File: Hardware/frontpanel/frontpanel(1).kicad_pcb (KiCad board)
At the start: 2 copper layers, 91.3 x 128.5 mm, 42 parts

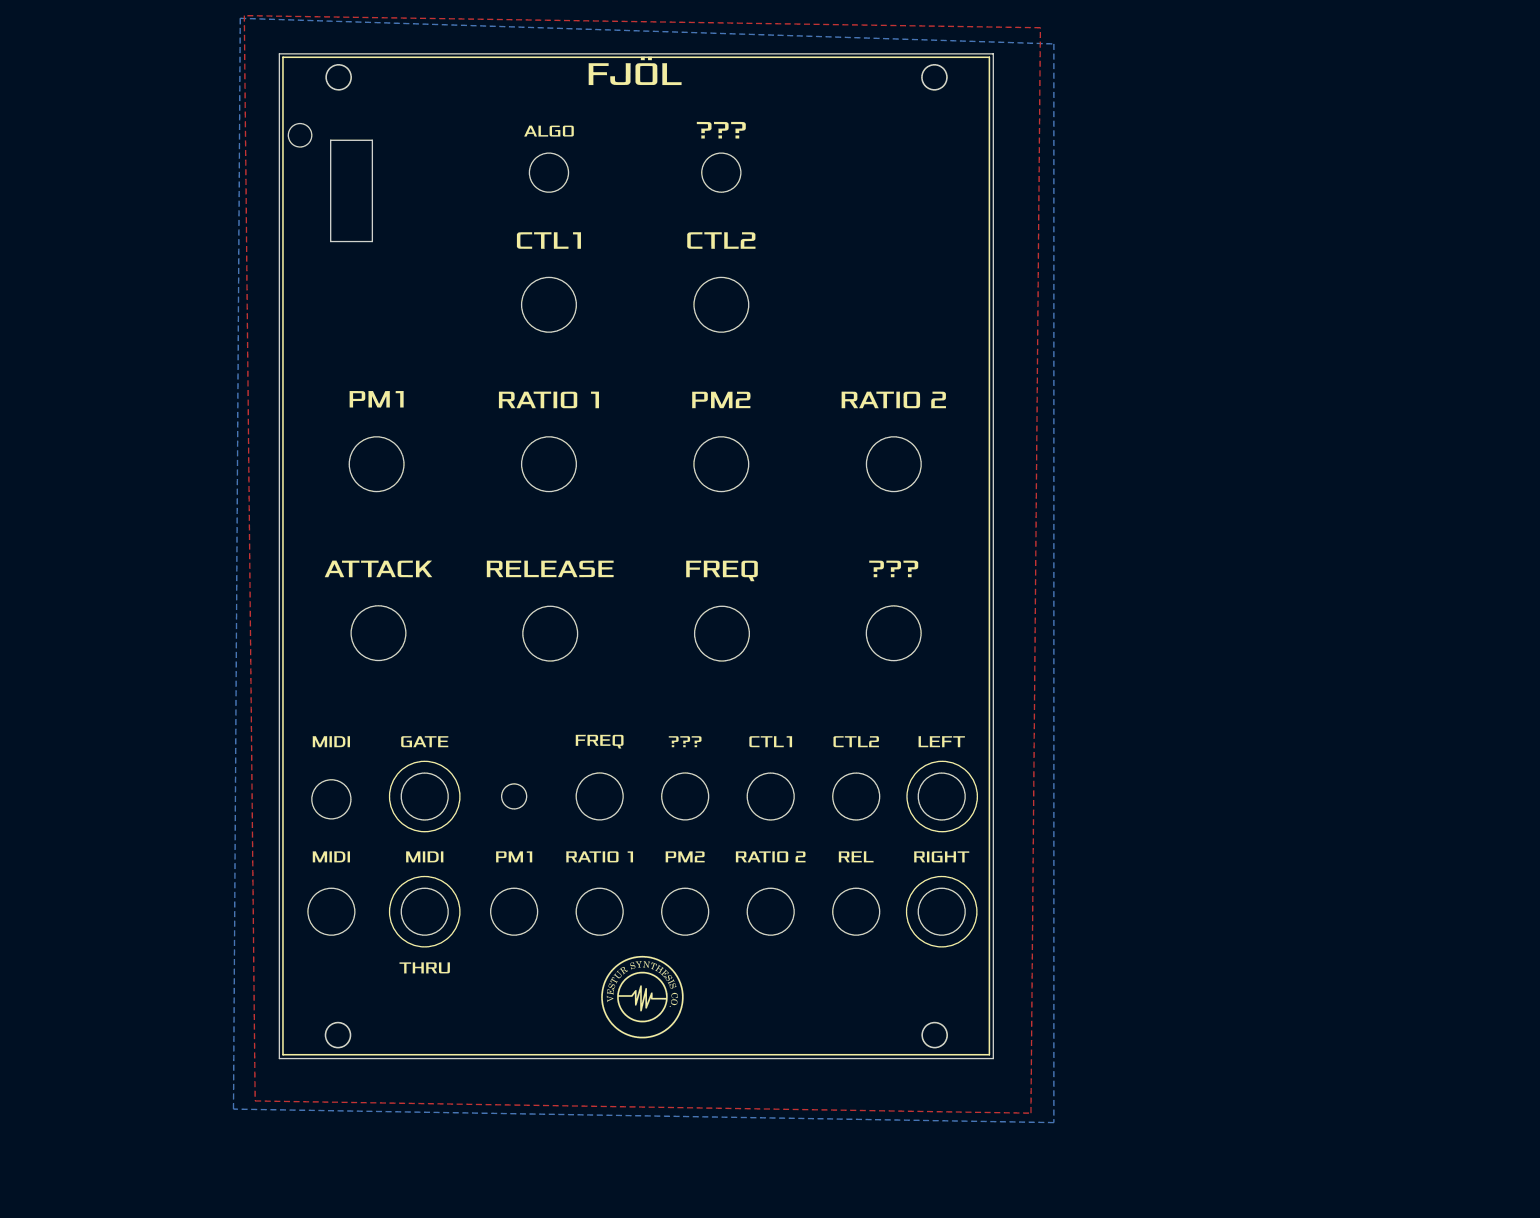
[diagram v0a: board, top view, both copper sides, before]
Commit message: upload everything
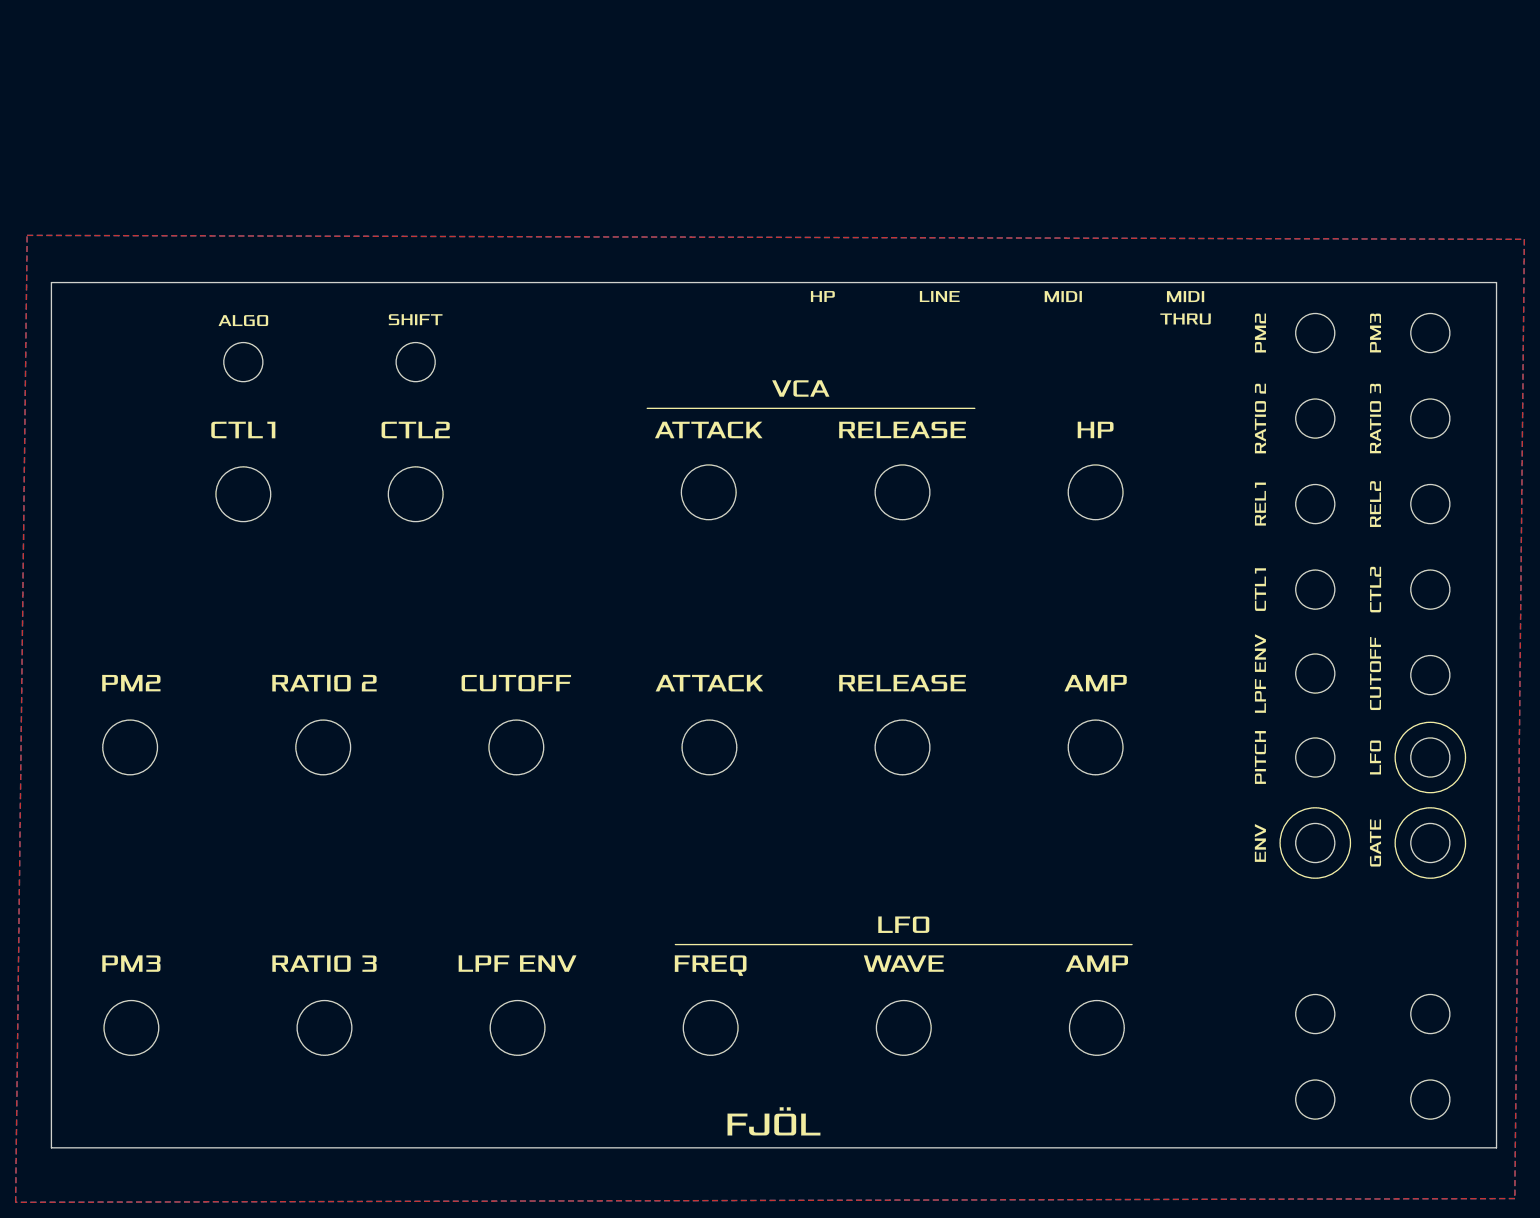
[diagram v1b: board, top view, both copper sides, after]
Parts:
- removed the G*** at (176.1, 113.2)
- removed the G*** at (170.0, 76.4)
- removed the G*** at (176.1, 98.5)
- removed the G*** at (137.9, 131.1)
- removed the G*** at (110.0, 113.2)
- removed the G*** at (121.4, 113.2)
- removed the G*** at (132.4, 113.2)
- removed the G*** at (165.2, 113.2)
- removed the G*** at (132.4, 98.5)
- removed the G*** at (103.8, 54.7)
- removed the G*** at (158.9, 45.6)
- removed the G*** at (158.9, 34.7)
- removed the G*** at (125.9, 54.8)
- removed the G*** at (158.9, 51.0)
- removed the G*** at (158.9, 40.2)
- added G***: LOGO, vestur-logo:line, F.Cu at (175.8, 41.6)
- added G***: LOGO, vestur-logo:cutoff, F.Cu at (121.7, 91.0)
- added G***: LOGO, vestur-logo:ratio3, F.Cu at (97.2, 126.9)
- added G***: LOGO, vestur-logo:rel2, F.Cu at (231.6, 68.1)
- added G***: LOGO, vestur-logo:lfo, F.Cu at (171.3, 121.9)
- added G***: LOGO, vestur-logo:ratio3-small, F.Cu at (231.6, 57.2)
- added G***: LOGO, vestur-logo:release, F.Cu at (171.1, 58.6)
- added G***: LOGO, vestur-logo:decay, F.Cu at (75.8, 69.8)
- added G***: LOGO, vestur-logo:amp, F.Cu at (195.8, 91.0)
- added G***: LOGO, vestur-logo:lfo-small, F.Cu at (231.6, 100.5)
- added G***: LOGO, vestur-logo:amp, F.Cu at (195.9, 126.9)
- added G***: LOGO, vestur-logo:filt-env-knob, F.Cu at (121.9, 126.9)
- added G***: LOGO, vestur-logo:pm3-small, F.Cu at (231.6, 46.3)
- added G***: LOGO, vestur-logo:wave, F.Cu at (171.2, 126.9)
- added G***: LOGO, vestur-logo:glide, F.Cu at (75.8, 75.4)
- added G***: LOGO, vestur-logo:cutoff-small, F.Cu at (231.6, 89.8)
- added G***: LOGO, vestur-logo:HP, F.Cu at (160.9, 41.6)
- added G***: LOGO, vestur-logo:vca, F.Cu at (158.1, 53.3)
- added G***: LOGO, vestur-logo:pm3, F.Cu at (72.5, 126.9)
- added G***: LOGO, vestur-logo:env, F.Cu at (216.9, 111.5)
- added G***: LOGO, vestur-logo:hp-knob, F.Cu at (195.8, 58.6)
- added G***: LOGO, vestur-logo:pitch, F.Cu at (216.9, 100.5)
- added G***: LOGO, vestur-logo:attack, F.Cu at (146.3, 58.6)
- added G***: LOGO, vestur-logo:rel1, F.Cu at (216.9, 68.1)
- added G***: LOGO, vestur-logo:decay-mirror, B.Cu at (75.8, 69.8)
- added G*** (x2): LOGO, vestur-logo:feedback-mirror, B.Cu at (119.9, 69.8)
- added G***: LOGO, vestur-logo:feedback2-mirror, B.Cu at (119.9, 75.3)
- added G***: LOGO, vestur-logo:det2-mirror, B.Cu at (119.9, 58.9)
- added G***: LOGO, vestur-logo:det3-mirror, B.Cu at (119.9, 64.4)
- added G***: LOGO, vestur-logo:glide-mirror, B.Cu at (75.8, 75.4)
- G***: footprint vestur-logo:???-small -> vestur-logo:filt-env-jack
- G***: footprint vestur-logo:pwm-solderm -> vestur-logo:feedback2
- G***: footprint vestur-logo:saw-solderm -> vestur-logo:det2
- G***: footprint vestur-logo:det-solderm -> vestur-logo:det3
- G***: footprint vestur-logo:square-solderm -> vestur-logo:feedback
- G***: footprint vestur-logo:??? -> vestur-logo:shift
- moved G*** 135.5 mm to (154.6, 147.1)
- moved G*** 130.7 mm to (207.3, 41.6)
- moved G*** 127.9 mm to (207.3, 44.5)
- moved G*** 122.3 mm to (231.6, 111.5), turned to 90 degrees
- moved G*** 109.6 mm to (191.6, 41.6)
- moved G*** 99.5 mm to (216.9, 46.3), turned to 90 degrees
- moved G*** 84.1 mm to (216.9, 57.2), turned to 90 degrees
- moved G*** 83.7 mm to (72.5, 91.0)
- moved G*** 81.3 mm to (97.2, 91.0)
- moved G*** 74.1 mm to (216.9, 89.8), turned to 90 degrees
- moved G*** 69.2 mm to (231.6, 79.1), turned to 90 degrees
- moved G*** 65.6 mm to (216.9, 79.1), turned to 90 degrees
- moved G*** 50.5 mm to (146.5, 127.2)
- moved G*** 47.4 mm to (171.1, 91.0)
- moved G*** 46.0 mm to (119.8, 75.3)
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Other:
- board size 91.3 x 128.5 mm -> 184.8 x 110.7 mm
